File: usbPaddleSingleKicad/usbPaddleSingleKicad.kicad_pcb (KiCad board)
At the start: 2 copper layers, 90 x 43 mm, 17 parts, among them U1 RP2040-ZERO, U2 RJ116P4C, U3 RJ116P4C, U4 RJ116P4C, U5 RJ116P4C

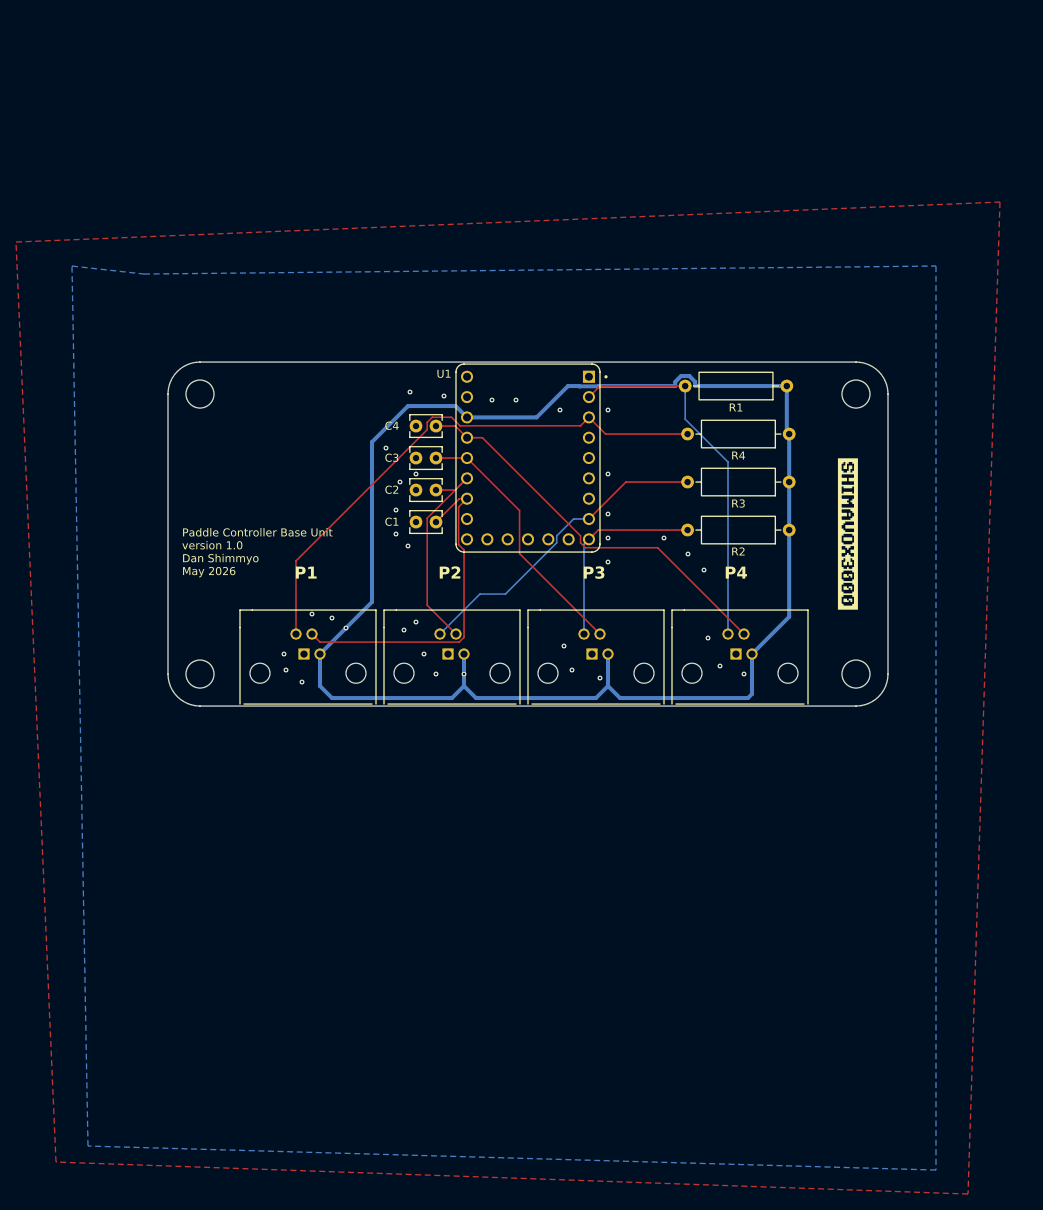
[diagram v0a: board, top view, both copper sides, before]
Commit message: new single paddle pcb
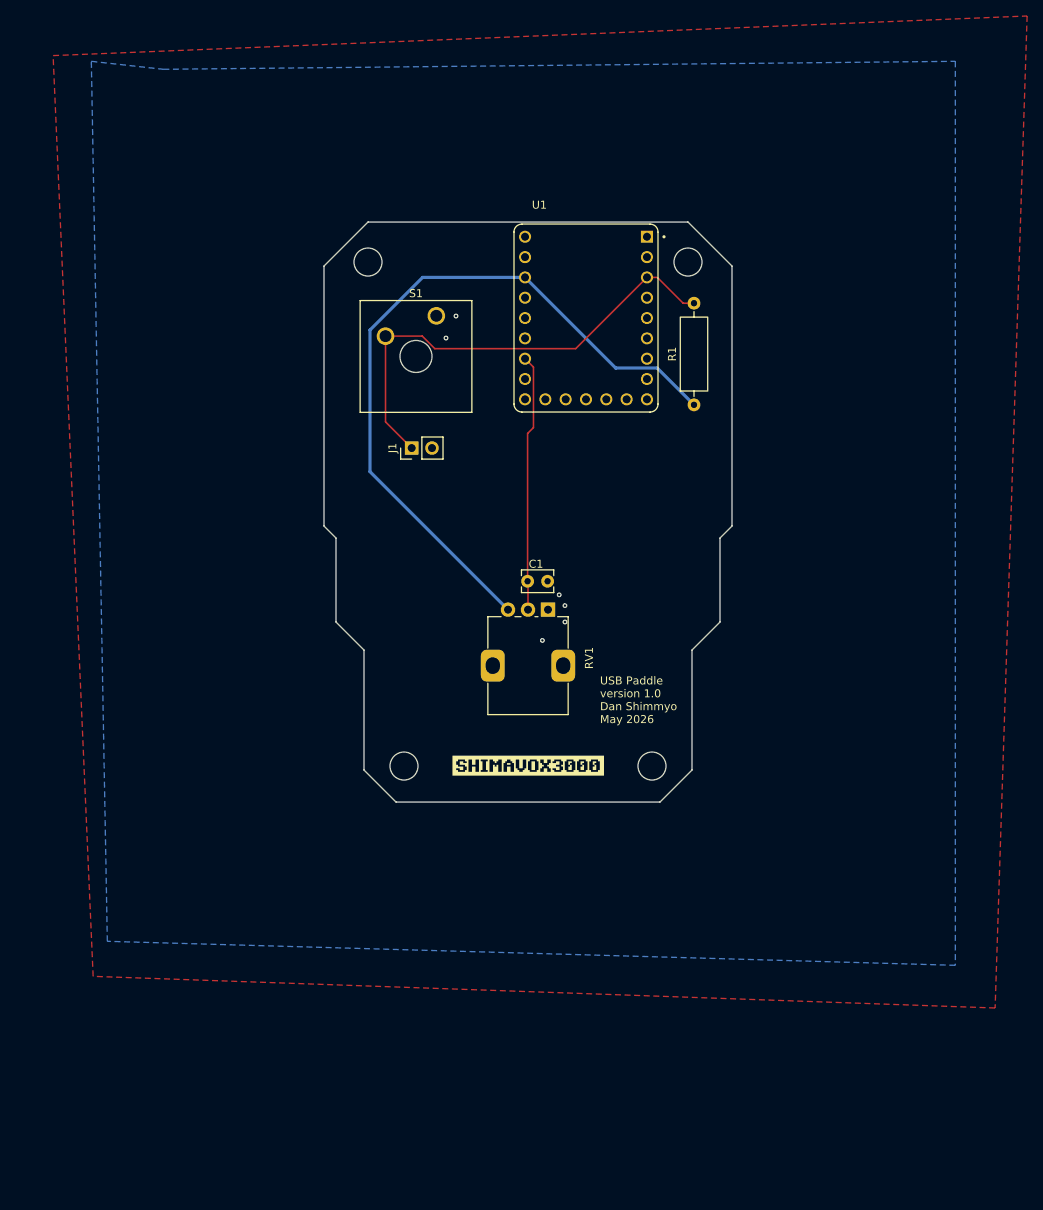
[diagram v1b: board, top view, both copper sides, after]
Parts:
- removed the ? at (95.6, 95.0)
- removed the ? at (177.6, 95.0)
- removed the ? at (95.6, 60.0)
- removed the ? at (177.6, 60.0)
- removed C2, C3, C4: .1µF, Capacitor_THT:C_Disc_D3.8mm_W2.6mm_P2.50mm
- removed R2, R3, R4: 10kΩ, Resistor_THT:R_Axial_DIN0309_L9.0mm_D3.2mm_P12.70mm_Horizontal
- removed U2, U3, U4, U5: RJ116P4C, RJ116P4C:RJ6P4C_GLX-N-64M
- added ?: , , F.Cu at (156.6, 43.5)
- added ?: , , F.Cu at (116.6, 43.5)
- added ?: , , F.Cu at (121.1, 106.5)
- added ?: , , F.Cu at (152.1, 106.5)
- added J1: Conn_01x02_Pin, Connector_PinHeader_2.54mm:PinHeader_1x02_P2.54mm_Vertical, F.Cu at (122.1, 66.7)
- added RV1: R_Potentiometer, Potentiometer_THT:Potentiometer_Alps_RK09K_Single_Vertical, F.Cu at (139.1, 86.9)
- added S1: ~, Button_Switch_Keyboard:SW_Cherry_MX_1.00u_Plate, F.Cu at (125.2, 50.2)
- moved U1 18.9 mm to (143.9, 50.5)
- moved C1 18.0 mm to (139.1, 83.4), turned to 180 degrees
- moved R1 11.8 mm to (157.4, 61.3), turned to 90 degrees
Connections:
- R1 pad 2: Net-(U1-GP1) -> Net-(J1-Pin_1)
- U1 pad 18: Net-(U1-GP27) -> unconnected-(U1-GP27-Pad18)
- U1 pad 19: Net-(U1-GP28) -> unconnected-(U1-GP28-Pad19)
- U1 pad 2: Net-(U1-GP1) -> unconnected-(U1-GP1-Pad2)
- U1 pad 20: Net-(U1-GP29) -> unconnected-(U1-GP29-Pad20)
- U1 pad 3: Net-(U1-GP2) -> Net-(J1-Pin_1)
- U1 pad 8: Net-(U1-GP7) -> unconnected-(U1-GP7-Pad8)
- U1 pad 9: Net-(U1-GP8) -> unconnected-(U1-GP8-Pad9)
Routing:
- net VCC: track 196.7 -> 91.9 mm, vias 2 -> 0
- net Net-(U1-GP2): track 67.8 -> 0.00 mm
- net Net-(J1-Pin_1): track 0.00 -> 59.6 mm
- net Net-(U1-GP29): track 49.8 -> 0.00 mm
- net Net-(U1-GP1): track 45.8 -> 0.00 mm
- net Net-(U1-GP7): track 39.3 -> 0.00 mm
- net Net-(U1-GP28): track 32.8 -> 0.00 mm
- net Net-(U1-GP27): track 27.5 -> 0.00 mm
- net Net-(U1-GP8): track 24.9 -> 0.00 mm
- net Net-(J2-Pin_2): track 42.8 -> 32.1 mm
- net GND: vias 34 -> 6
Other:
- board size 90 x 43 mm -> 51 x 72.5 mm
- board text added: "USB Paddle version 1.0 Dan Shimmyo May 2026"
- board text removed: "BTN"
- board text removed: "P1"
- board text removed: "P2"
- board text removed: "P3"
- board text removed: "P4"
- board text removed: "Paddle Controller Base Unit version 1.0 Dan Shimmyo May 2026"
